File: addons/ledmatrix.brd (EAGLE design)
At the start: 30.5 x 25.4 mm, 11 parts

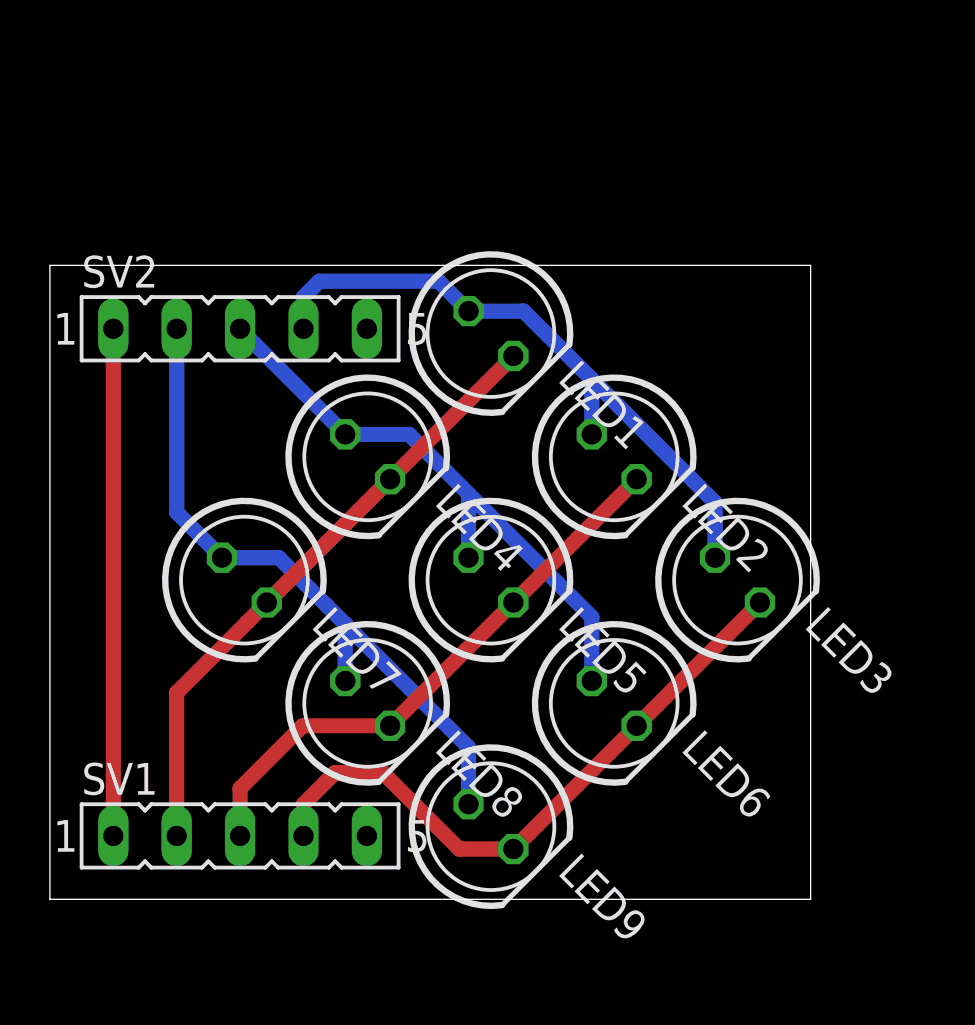
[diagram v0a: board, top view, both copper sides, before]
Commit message: anpassen an neues board
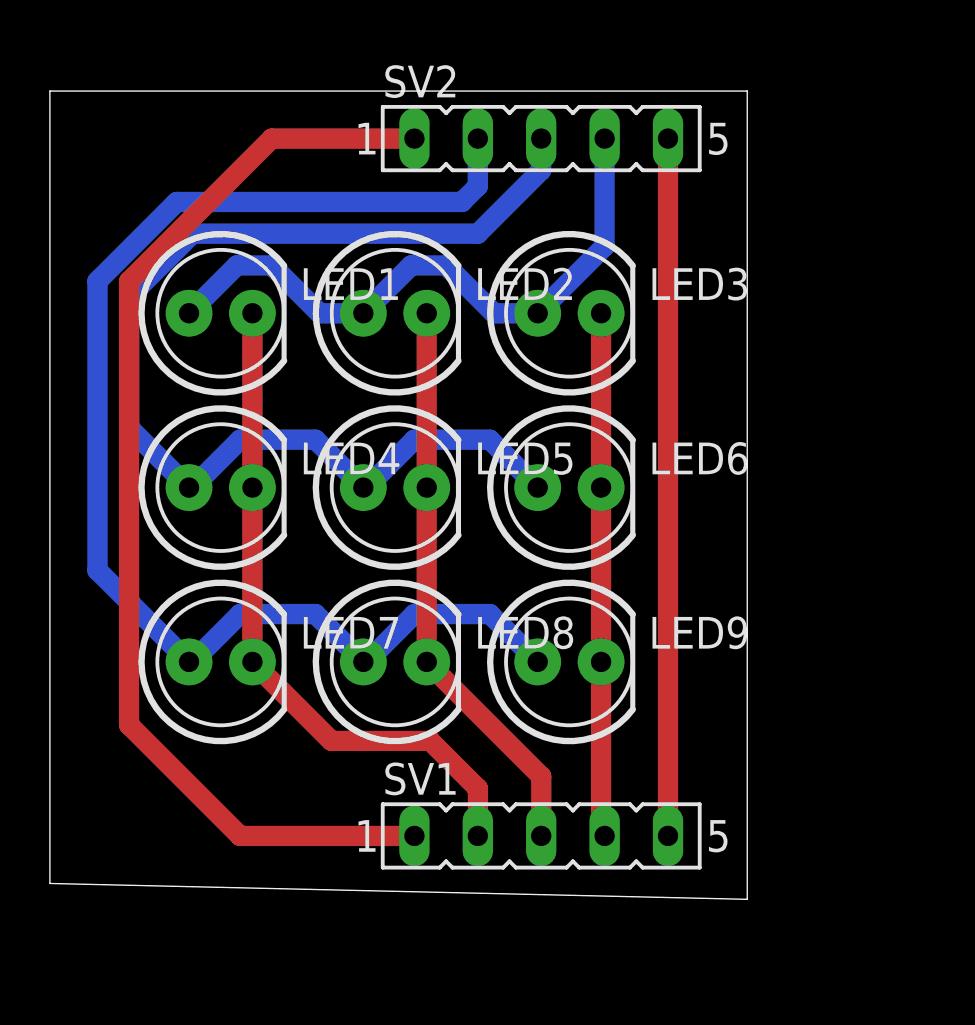
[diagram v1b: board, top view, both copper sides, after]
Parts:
- LED1, LED2, LED3, LED4, LED5, LED6, LED7, LED8, LED9: device led:LED5MM -> SparkFun:LED5MM
- moved SV2 14.3 mm to (19.7, 30.5)
- moved LED3 12.6 mm to (20.8, 23.5), turned to 0 degrees
- moved SV1 12.1 mm to (19.7, 2.54)
- moved LED1 10.9 mm to (6.84, 23.5), turned to 0 degrees
- moved LED2 10.5 mm to (13.8, 23.5), turned to 0 degrees
- moved LED6 8.83 mm to (20.8, 16.5), turned to 0 degrees
- moved LED9 7.31 mm to (20.8, 9.51), turned to 0 degrees
- moved LED4 6.02 mm to (6.84, 16.5), turned to 0 degrees
- moved LED5 5.34 mm to (13.8, 16.5), turned to 0 degrees
- moved LED7 3.41 mm to (6.84, 9.51), turned to 0 degrees
- moved LED8 1.99 mm to (13.8, 9.51), turned to 0 degrees
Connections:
- net PD2 renamed PC5
- net PD3 renamed PC4
- net PD4 renamed PB2
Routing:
- net GND: track 0.00 -> 27.9 mm
- net PD5: track 27.5 -> 52.6 mm
- net VCC: track 20.3 -> 44.8 mm
- net PD6: track 24.0 -> 45.7 mm
- net PC5: track 31.8 -> 27.0 mm
- net PB2: track 25.4 -> 20.8 mm
- net PD7: track 26.1 -> 25.3 mm
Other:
- board size 30.5 x 25.4 mm -> 27.9 x 32.4 mm
